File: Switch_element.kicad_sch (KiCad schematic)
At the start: 24 parts, among them IC301 TPS259802ONRGER, IC302 TPS259802ONRGER

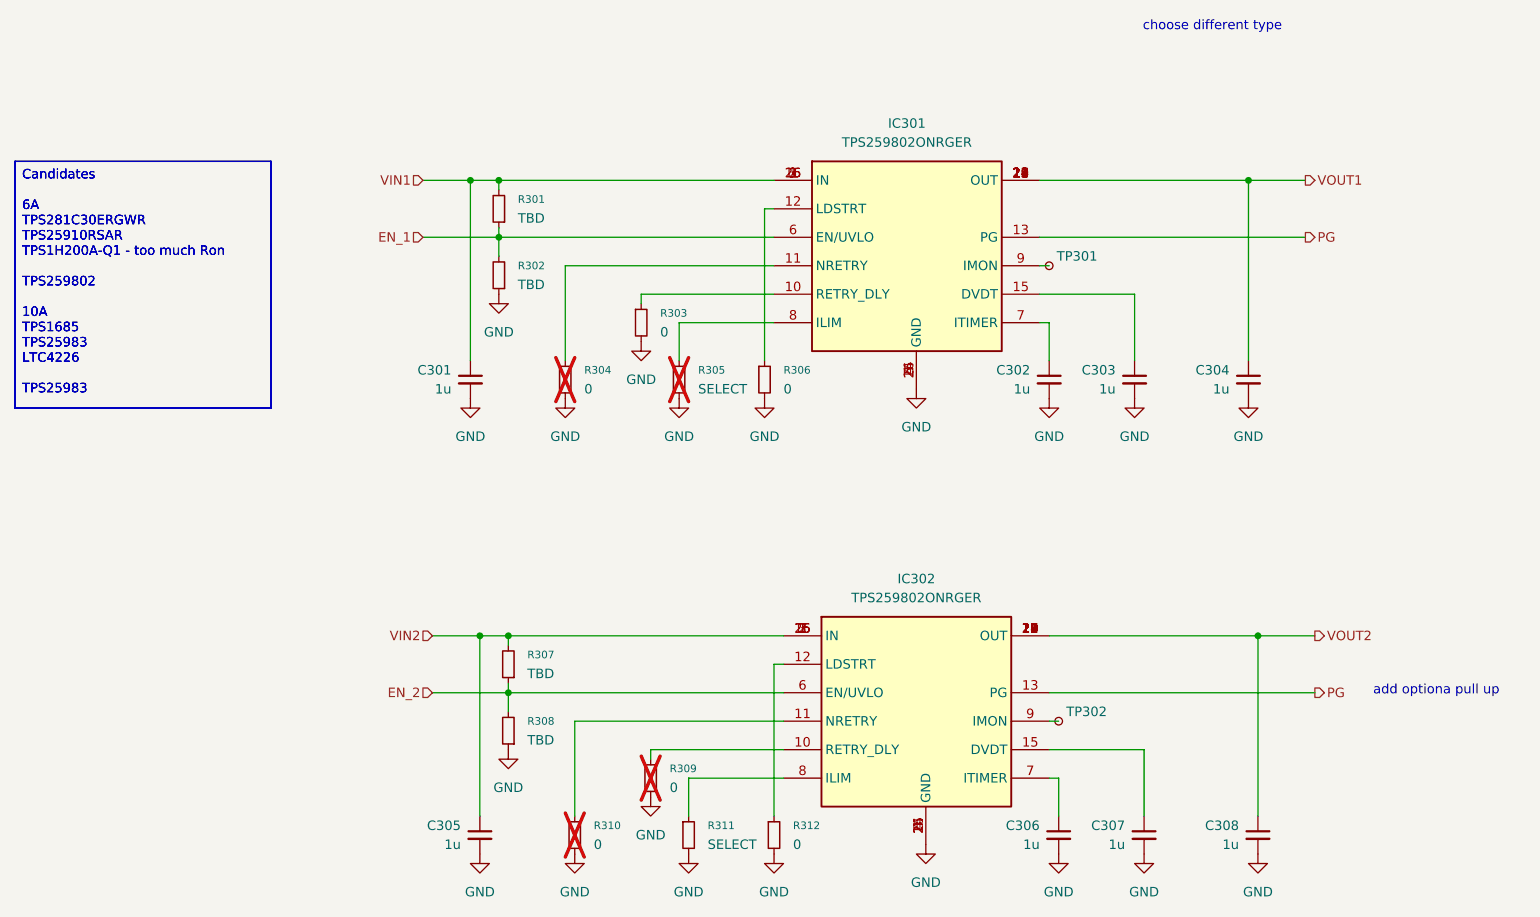
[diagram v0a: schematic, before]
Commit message: small changes to test board
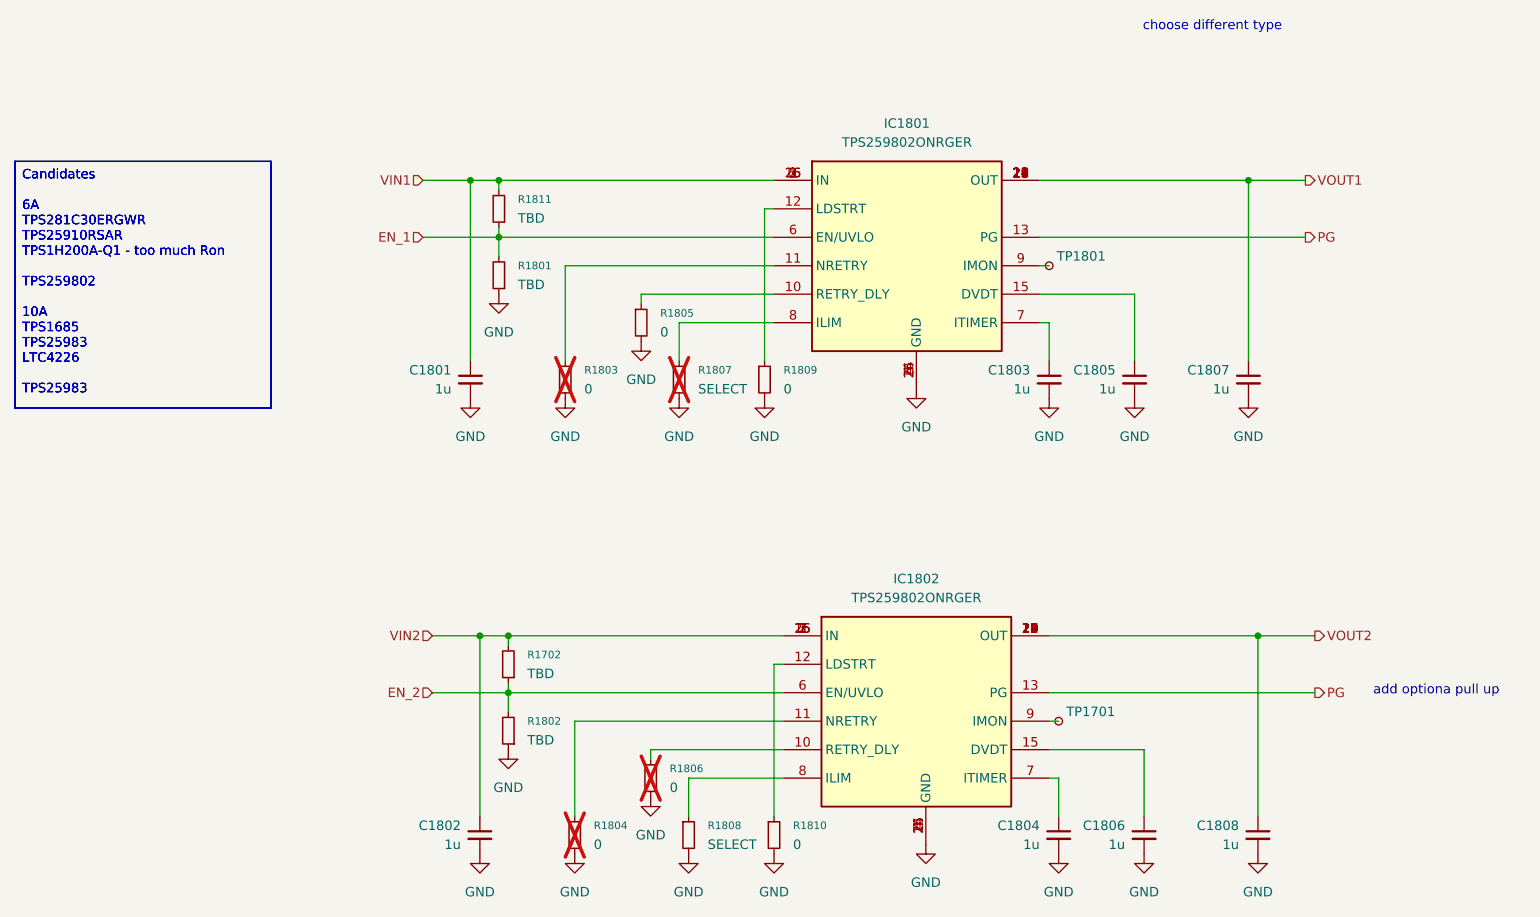
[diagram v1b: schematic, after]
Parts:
- renumbered C301 to C1801, C305 to C1802, C302 to C1803, C306 to C1804, C303 to C1805, C307 to C1806, C304 to C1807, C308 to C1808, IC301 to IC1801, IC302 to IC1802, R307 to R1702, R302 to R1801, R308 to R1802, R304 to R1803, R310 to R1804, R303 to R1805, R309 to R1806, R305 to R1807, R311 to R1808, R306 to R1809, R312 to R1810, R301 to R1811, TP302 to TP1701, TP301 to TP1801
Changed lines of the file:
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@@
 		(on_board yes)
 		(dnp no)
-		(property "Reference" "C302"
+		(property "Reference" "C1803"
 			(at 180.34 67.3162 0)
 			(effects
@@
 		(on_board yes)
 		(dnp no)
-		(property "Reference" "TP301"
+		(property "Reference" "TP1801"
 			(at 183.896 52.0699 0)
 			(effects
@@
 		(dnp no)
 		(fields_autoplaced yes)
-		(property "Reference" "#PWR0146"
+		(property "Reference" "#PWR01813"
 			(at 165.1 76.2 0)
 			(effects
@@
 		(dnp no)
 		(fields_autoplaced yes)
-		(property "Reference" "#PWR0149"
+		(property "Reference" "#PWR01804"
 			(at 110.49 124.46 0)
 			(effects
@@
 		(on_board yes)
 		(dnp no)
-		(property "Reference" "C301"
+		(property "Reference" "C1801"
 			(at 102.87 67.3162 0)
 			(effects
@@
 		(dnp no)
 		(fields_autoplaced yes)
-		(property "Reference" "#PWR0145"
+		(property "Reference" "#PWR01819"
 			(at 209.55 77.47 0)
 			(effects
@@
 		(dnp no)
 		(fields_autoplaced yes)
-		(property "Reference" "R302"
+		(property "Reference" "R1801"
 			(at 111.76 53.3399 0)
 			(effects
@@
 		(dnp no)
 		(fields_autoplaced yes)
-		(property "Reference" "#PWR0139"
+		(property "Reference" "#PWR01801"
 			(at 105.41 77.47 0)
 			(effects
@@
 		(dnp no)
 		(fields_autoplaced yes)
-		(property "Reference" "IC302"
+		(property "Reference" "IC1802"
 			(at 165.1 95.25 0)
 			(effects
@@
 		(dnp no)
 		(fields_autoplaced yes)
-		(property "Reference" "#PWR0142"
+		(property "Reference" "#PWR01811"
 			(at 144.78 77.47 0)
 			(effects
@@
 		(dnp yes)
 		(fields_autoplaced yes)
-		(property "Reference" "R310"
+		(property "Reference" "R1804"
 			(at 121.92 128.2699 0)
 			(effects
@@
 		(on_board yes)
 		(dnp no)
-		(property "Reference" "C303"
+		(property "Reference" "C1805"
 			(at 191.77 67.3162 0)
 			(effects
@@
 		(dnp no)
 		(fields_autoplaced yes)
-		(property "Reference" "#PWR0147"
+		(property "Reference" "#PWR01817"
 			(at 194.31 77.47 0)
 			(effects
@@
 		(dnp no)
 		(fields_autoplaced yes)
-		(property "Reference" "#PWR0140"
+		(property "Reference" "#PWR01803"
 			(at 109.22 63.5 0)
 			(effects
@@
 		(on_board yes)
 		(dnp no)
-		(property "Reference" "C304"
+		(property "Reference" "C1807"
 			(at 207.01 67.3162 0)
 			(effects
@@
 		(dnp no)
 		(fields_autoplaced yes)
-		(property "Reference" "R306"
+		(property "Reference" "R1809"
 			(at 147.32 67.3099 0)
 			(effects
@@
 		(on_board yes)
 		(dnp no)
-		(property "Reference" "TP302"
+		(property "Reference" "TP1701"
 			(at 185.166 113.0299 0)
 			(effects
@@
 		(dnp no)
 		(fields_autoplaced yes)
-		(property "Reference" "R311"
+		(property "Reference" "R1808"
 			(at 137.16 128.2699 0)
 			(effects
@@
 		(on_board yes)
 		(dnp no)
-		(property "Reference" "C306"
+		(property "Reference" "C1804"
 			(at 181.61 128.2762 0)
 			(effects
@@
 		(on_board yes)
 		(dnp no)
-		(property "Reference" "C308"
+		(property "Reference" "C1808"
 			(at 208.28 128.2762 0)
 			(effects
@@
 		(dnp yes)
 		(fields_autoplaced yes)
-		(property "Reference" "R304"
+		(property "Reference" "R1803"
 			(at 120.65 67.3099 0)
 			(effects
@@
 		(dnp no)
 		(fields_autoplaced yes)
-		(property "Reference" "#PWR0155"
+		(property "Reference" "#PWR01814"
 			(at 166.37 137.16 0)
 			(effects
@@
 		(dnp no)
 		(fields_autoplaced yes)
-		(property "Reference" "#PWR0156"
+		(property "Reference" "#PWR01818"
 			(at 195.58 138.43 0)
 			(effects
@@
 		(dnp no)
 		(fields_autoplaced yes)
-		(property "Reference" "#PWR0153"
+		(property "Reference" "#PWR01808"
 			(at 129.54 130.81 0)
 			(effects
@@
 		(dnp no)
 		(fields_autoplaced yes)
-		(property "Reference" "R308"
+		(property "Reference" "R1802"
 			(at 113.03 114.2999 0)
 			(effects
@@
 		(dnp no)
 		(fields_autoplaced yes)
-		(property "Reference" "#PWR0150"
+		(property "Reference" "#PWR01810"
 			(at 134.62 138.43 0)
 			(effects
@@
 		(on_board yes)
 		(dnp no)
-		(property "Reference" "C305"
+		(property "Reference" "C1802"
 			(at 104.14 128.2762 0)
 			(effects
@@
 		(dnp yes)
 		(fields_autoplaced yes)
-		(property "Reference" "R305"
+		(property "Reference" "R1807"
 			(at 135.89 67.3099 0)
 			(effects
@@
 		(dnp no)
 		(fields_autoplaced yes)
-		(property "Reference" "#PWR0151"
+		(property "Reference" "#PWR01802"
 			(at 106.68 138.43 0)
 			(effects
@@
 		(dnp no)
 		(fields_autoplaced yes)
-		(property "Reference" "R303"
+		(property "Reference" "R1805"
 			(at 130.81 59.6899 0)
 			(effects
@@
 		(dnp no)
 		(fields_autoplaced yes)
-		(property "Reference" "#PWR0157"
+		(property "Reference" "#PWR01816"
 			(at 184.15 138.43 0)
 			(effects
@@
 		(dnp no)
 		(fields_autoplaced yes)
-		(property "Reference" "#PWR0143"
+		(property "Reference" "#PWR01807"
 			(at 128.27 69.85 0)
 			(effects
@@
 		(dnp no)
 		(fields_autoplaced yes)
-		(property "Reference" "#PWR0158"
+		(property "Reference" "#PWR01820"
 			(at 210.82 138.43 0)
 			(effects
@@
 		(dnp no)
 		(fields_autoplaced yes)
-		(property "Reference" "IC301"
+		(property "Reference" "IC1801"
 			(at 163.83 34.29 0)
 			(effects
@@
 		(dnp no)
 		(fields_autoplaced yes)
-		(property "Reference" "#PWR0152"
+		(property "Reference" "#PWR01806"
 			(at 119.38 138.43 0)
 			(effects
@@
 		(dnp no)
 		(fields_autoplaced yes)
-		(property "Reference" "#PWR0141"
+		(property "Reference" "#PWR01809"
 			(at 133.35 77.47 0)
 			(effects
@@
 		(dnp no)
 		(fields_autoplaced yes)
-		(property "Reference" "R301"
+		(property "Reference" "R1811"
 			(at 111.76 44.4499 0)
 			(effects
@@
 		(dnp no)
 		(fields_autoplaced yes)
-		(property "Reference" "#PWR0154"
+		(property "Reference" "#PWR01812"
 			(at 146.05 138.43 0)
 			(effects
@@
 		(on_board yes)
 		(dnp no)
-		(property "Reference" "C307"
+		(property "Reference" "C1806"
 			(at 193.04 128.2762 0)
 			(effects
@@
 		(dnp yes)
 		(fields_autoplaced yes)
-		(property "Reference" "R309"
+		(property "Reference" "R1806"
 			(at 132.08 120.6499 0)
 			(effects
@@
 		(dnp no)
 		(fields_autoplaced yes)
-		(property "Reference" "#PWR0144"
+		(property "Reference" "#PWR01805"
 			(at 118.11 77.47 0)
 			(effects
@@
 		(dnp no)
 		(fields_autoplaced yes)
-		(property "Reference" "R312"
+		(property "Reference" "R1810"
 			(at 148.59 128.2699 0)
 			(effects
@@
 		(dnp no)
 		(fields_autoplaced yes)
-		(property "Reference" "R307"
+		(property "Reference" "R1702"
 			(at 113.03 105.4099 0)
 			(effects
@@
 		(dnp no)
 		(fields_autoplaced yes)
-		(property "Reference" "#PWR0148"
+		(property "Reference" "#PWR01815"
 			(at 182.88 77.47 0)
 			(effects

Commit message: nearly finnished CORE pcb
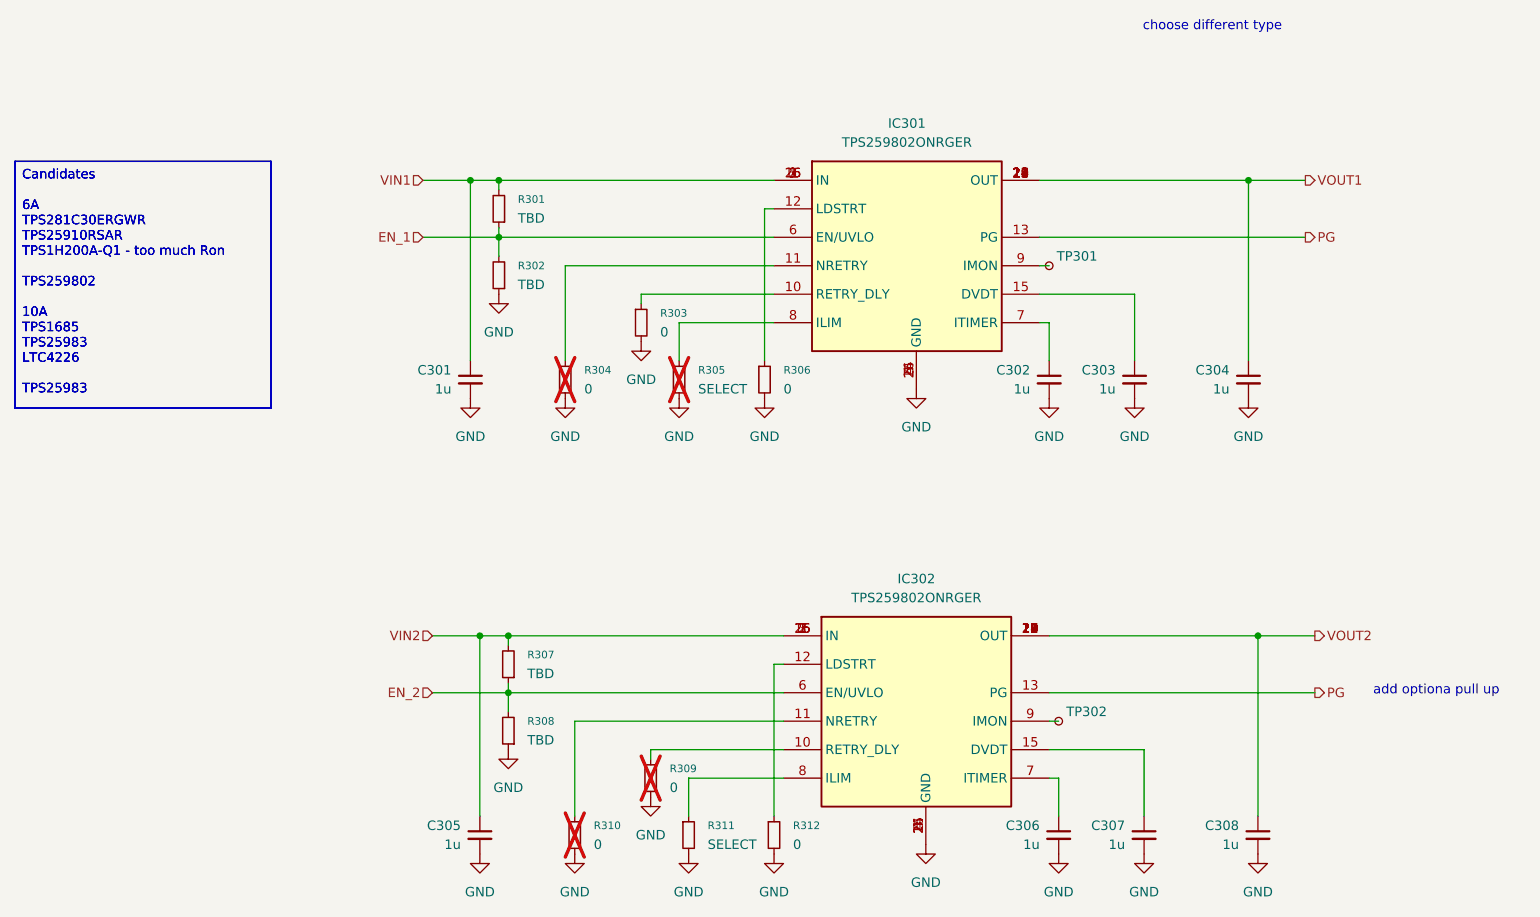
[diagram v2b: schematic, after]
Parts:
- renumbered C1801 to C301, C1803 to C302, C1805 to C303, C1807 to C304, C1802 to C305, C1804 to C306, C1806 to C307, C1808 to C308, IC1801 to IC301, IC1802 to IC302, R1811 to R301, R1801 to R302, R1805 to R303, R1803 to R304, R1807 to R305, R1809 to R306, R1702 to R307, R1802 to R308, R1806 to R309, R1804 to R310, R1808 to R311, R1810 to R312, TP1801 to TP301, TP1701 to TP302
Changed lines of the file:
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@@
 		(on_board yes)
 		(dnp no)
-		(property "Reference" "C1803"
+		(property "Reference" "C302"
 			(at 180.34 67.3162 0)
 			(effects
@@
 		(on_board yes)
 		(dnp no)
-		(property "Reference" "TP1801"
+		(property "Reference" "TP301"
 			(at 183.896 52.0699 0)
 			(effects
@@
 		(dnp no)
 		(fields_autoplaced yes)
-		(property "Reference" "#PWR01813"
+		(property "Reference" "#PWR0146"
 			(at 165.1 76.2 0)
 			(effects
@@
 		(dnp no)
 		(fields_autoplaced yes)
-		(property "Reference" "#PWR01804"
+		(property "Reference" "#PWR0149"
 			(at 110.49 124.46 0)
 			(effects
@@
 		(on_board yes)
 		(dnp no)
-		(property "Reference" "C1801"
+		(property "Reference" "C301"
 			(at 102.87 67.3162 0)
 			(effects
@@
 		(dnp no)
 		(fields_autoplaced yes)
-		(property "Reference" "#PWR01819"
+		(property "Reference" "#PWR0145"
 			(at 209.55 77.47 0)
 			(effects
@@
 		(dnp no)
 		(fields_autoplaced yes)
-		(property "Reference" "R1801"
+		(property "Reference" "R302"
 			(at 111.76 53.3399 0)
 			(effects
@@
 		(dnp no)
 		(fields_autoplaced yes)
-		(property "Reference" "#PWR01801"
+		(property "Reference" "#PWR0139"
 			(at 105.41 77.47 0)
 			(effects
@@
 		(dnp no)
 		(fields_autoplaced yes)
-		(property "Reference" "IC1802"
+		(property "Reference" "IC302"
 			(at 165.1 95.25 0)
 			(effects
@@
 		(dnp no)
 		(fields_autoplaced yes)
-		(property "Reference" "#PWR01811"
+		(property "Reference" "#PWR0142"
 			(at 144.78 77.47 0)
 			(effects
@@
 		(dnp yes)
 		(fields_autoplaced yes)
-		(property "Reference" "R1804"
+		(property "Reference" "R310"
 			(at 121.92 128.2699 0)
 			(effects
@@
 		(on_board yes)
 		(dnp no)
-		(property "Reference" "C1805"
+		(property "Reference" "C303"
 			(at 191.77 67.3162 0)
 			(effects
@@
 		(dnp no)
 		(fields_autoplaced yes)
-		(property "Reference" "#PWR01817"
+		(property "Reference" "#PWR0147"
 			(at 194.31 77.47 0)
 			(effects
@@
 		(dnp no)
 		(fields_autoplaced yes)
-		(property "Reference" "#PWR01803"
+		(property "Reference" "#PWR0140"
 			(at 109.22 63.5 0)
 			(effects
@@
 		(on_board yes)
 		(dnp no)
-		(property "Reference" "C1807"
+		(property "Reference" "C304"
 			(at 207.01 67.3162 0)
 			(effects
@@
 		(dnp no)
 		(fields_autoplaced yes)
-		(property "Reference" "R1809"
+		(property "Reference" "R306"
 			(at 147.32 67.3099 0)
 			(effects
@@
 		(on_board yes)
 		(dnp no)
-		(property "Reference" "TP1701"
+		(property "Reference" "TP302"
 			(at 185.166 113.0299 0)
 			(effects
@@
 		(dnp no)
 		(fields_autoplaced yes)
-		(property "Reference" "R1808"
+		(property "Reference" "R311"
 			(at 137.16 128.2699 0)
 			(effects
@@
 		(on_board yes)
 		(dnp no)
-		(property "Reference" "C1804"
+		(property "Reference" "C306"
 			(at 181.61 128.2762 0)
 			(effects
@@
 		(on_board yes)
 		(dnp no)
-		(property "Reference" "C1808"
+		(property "Reference" "C308"
 			(at 208.28 128.2762 0)
 			(effects
@@
 		(dnp yes)
 		(fields_autoplaced yes)
-		(property "Reference" "R1803"
+		(property "Reference" "R304"
 			(at 120.65 67.3099 0)
 			(effects
@@
 		(dnp no)
 		(fields_autoplaced yes)
-		(property "Reference" "#PWR01814"
+		(property "Reference" "#PWR0155"
 			(at 166.37 137.16 0)
 			(effects
@@
 		(dnp no)
 		(fields_autoplaced yes)
-		(property "Reference" "#PWR01818"
+		(property "Reference" "#PWR0156"
 			(at 195.58 138.43 0)
 			(effects
@@
 		(dnp no)
 		(fields_autoplaced yes)
-		(property "Reference" "#PWR01808"
+		(property "Reference" "#PWR0153"
 			(at 129.54 130.81 0)
 			(effects
@@
 		(dnp no)
 		(fields_autoplaced yes)
-		(property "Reference" "R1802"
+		(property "Reference" "R308"
 			(at 113.03 114.2999 0)
 			(effects
@@
 		(dnp no)
 		(fields_autoplaced yes)
-		(property "Reference" "#PWR01810"
+		(property "Reference" "#PWR0150"
 			(at 134.62 138.43 0)
 			(effects
@@
 		(on_board yes)
 		(dnp no)
-		(property "Reference" "C1802"
+		(property "Reference" "C305"
 			(at 104.14 128.2762 0)
 			(effects
@@
 		(dnp yes)
 		(fields_autoplaced yes)
-		(property "Reference" "R1807"
+		(property "Reference" "R305"
 			(at 135.89 67.3099 0)
 			(effects
@@
 		(dnp no)
 		(fields_autoplaced yes)
-		(property "Reference" "#PWR01802"
+		(property "Reference" "#PWR0151"
 			(at 106.68 138.43 0)
 			(effects
@@
 		(dnp no)
 		(fields_autoplaced yes)
-		(property "Reference" "R1805"
+		(property "Reference" "R303"
 			(at 130.81 59.6899 0)
 			(effects
@@
 		(dnp no)
 		(fields_autoplaced yes)
-		(property "Reference" "#PWR01816"
+		(property "Reference" "#PWR0157"
 			(at 184.15 138.43 0)
 			(effects
@@
 		(dnp no)
 		(fields_autoplaced yes)
-		(property "Reference" "#PWR01807"
+		(property "Reference" "#PWR0143"
 			(at 128.27 69.85 0)
 			(effects
@@
 		(dnp no)
 		(fields_autoplaced yes)
-		(property "Reference" "#PWR01820"
+		(property "Reference" "#PWR0158"
 			(at 210.82 138.43 0)
 			(effects
@@
 		(dnp no)
 		(fields_autoplaced yes)
-		(property "Reference" "IC1801"
+		(property "Reference" "IC301"
 			(at 163.83 34.29 0)
 			(effects
@@
 		(dnp no)
 		(fields_autoplaced yes)
-		(property "Reference" "#PWR01806"
+		(property "Reference" "#PWR0152"
 			(at 119.38 138.43 0)
 			(effects
@@
 		(dnp no)
 		(fields_autoplaced yes)
-		(property "Reference" "#PWR01809"
+		(property "Reference" "#PWR0141"
 			(at 133.35 77.47 0)
 			(effects
@@
 		(dnp no)
 		(fields_autoplaced yes)
-		(property "Reference" "R1811"
+		(property "Reference" "R301"
 			(at 111.76 44.4499 0)
 			(effects
@@
 		(dnp no)
 		(fields_autoplaced yes)
-		(property "Reference" "#PWR01812"
+		(property "Reference" "#PWR0154"
 			(at 146.05 138.43 0)
 			(effects
@@
 		(on_board yes)
 		(dnp no)
-		(property "Reference" "C1806"
+		(property "Reference" "C307"
 			(at 193.04 128.2762 0)
 			(effects
@@
 		(dnp yes)
 		(fields_autoplaced yes)
-		(property "Reference" "R1806"
+		(property "Reference" "R309"
 			(at 132.08 120.6499 0)
 			(effects
@@
 		(dnp no)
 		(fields_autoplaced yes)
-		(property "Reference" "#PWR01805"
+		(property "Reference" "#PWR0144"
 			(at 118.11 77.47 0)
 			(effects
@@
 		(dnp no)
 		(fields_autoplaced yes)
-		(property "Reference" "R1810"
+		(property "Reference" "R312"
 			(at 148.59 128.2699 0)
 			(effects
@@
 		(dnp no)
 		(fields_autoplaced yes)
-		(property "Reference" "R1702"
+		(property "Reference" "R307"
 			(at 113.03 105.4099 0)
 			(effects
@@
 		(dnp no)
 		(fields_autoplaced yes)
-		(property "Reference" "#PWR01815"
+		(property "Reference" "#PWR0148"
 			(at 182.88 77.47 0)
 			(effects
